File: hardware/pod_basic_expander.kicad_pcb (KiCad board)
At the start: 2 copper layers, 45 x 44 mm, 7 parts, among them J1 POD, SW1 SW_Push, SW2 SW_Push, SW3 SW_Push, SW4 SW_Push

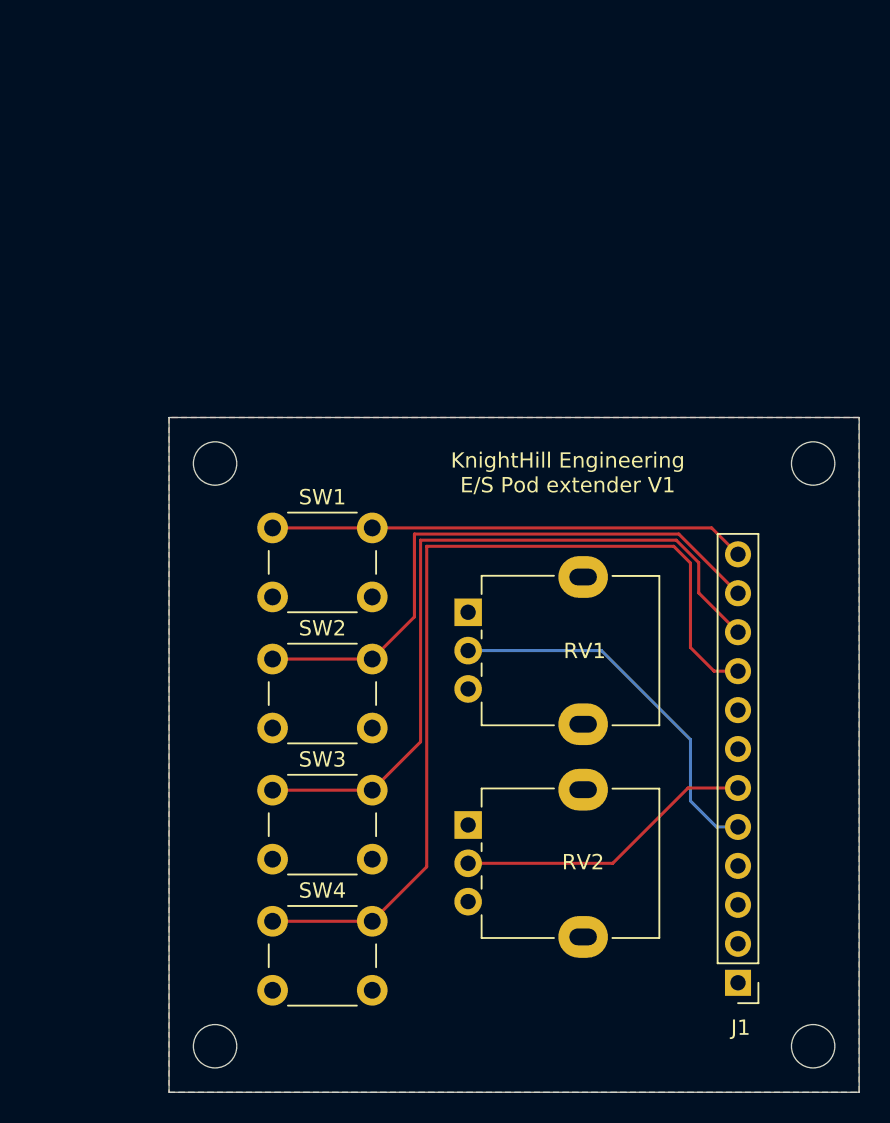
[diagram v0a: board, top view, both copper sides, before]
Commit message: pcd changes
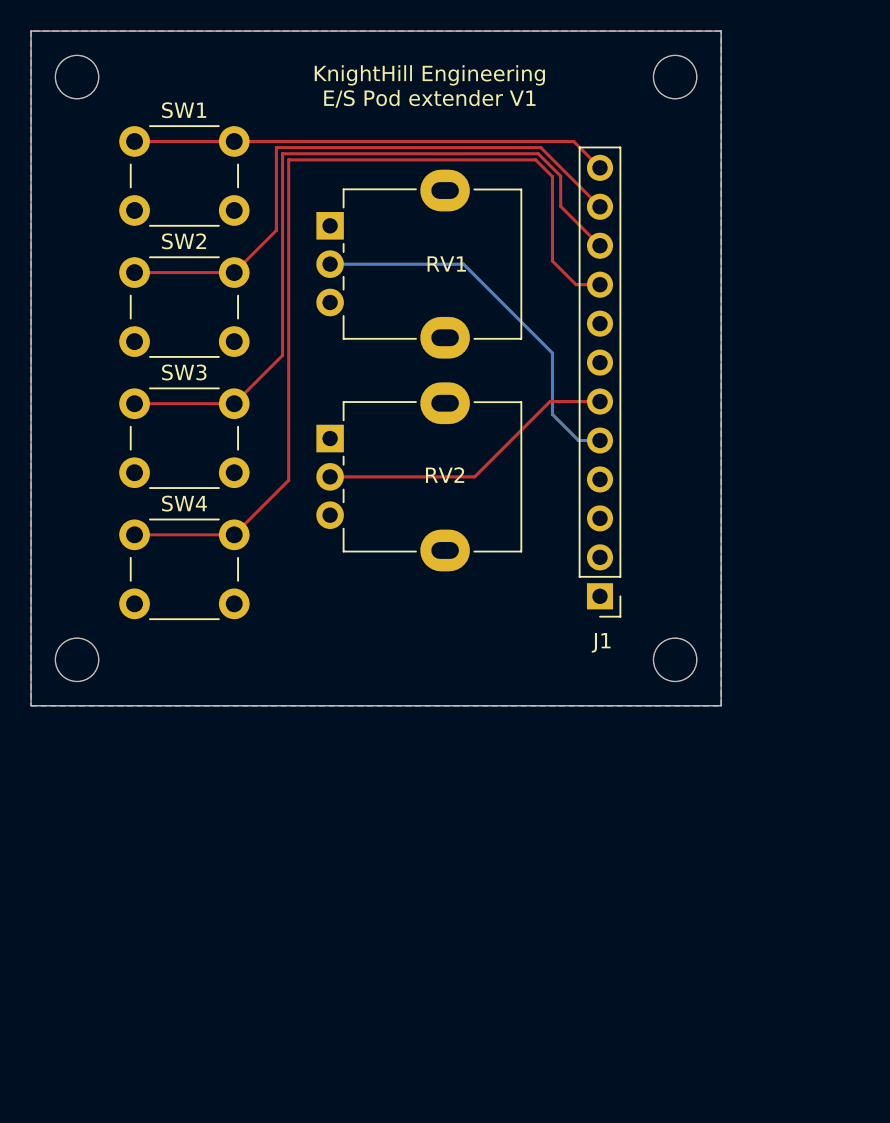
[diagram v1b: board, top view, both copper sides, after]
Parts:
- moved J1 26.8 mm to (101.1, 77.7)
- moved RV1 26.8 mm to (83.5, 53.5)
- moved SW1 26.8 mm to (70.8, 48.0)
- moved SW2 26.8 mm to (70.8, 56.5)
- moved SW3 26.8 mm to (70.8, 65.1)
- moved RV2 26.8 mm to (83.5, 67.4)
- moved SW4 26.8 mm to (70.8, 73.7)
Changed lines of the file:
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@@
   (net 12 "/D7")
   (footprint "Potentiometer_THT:Potentiometer_Alpha_RD901F-40-00D_Single_Vertical" (layer "F.Cu")
-    (at 92.5 92.57)
+    (at 83.5 67.37)
     (descr "Potentiometer, vertical, 9mm, single, http://www.taiwanalpha.com.tw/downloads?target=products&id=113")
     (tags "potentiometer vertical 9mm single")
@@
   )
   (footprint "Button_Switch_THT:SW_PUSH_6mm" (layer "F.Cu")
-    (at 79.75 81.75)
+    (at 70.75 56.55)
     (descr "https://www.omron.com/ecb/products/pdf/en-b3f.pdf")
     (tags "tact sw push 6mm")
@@
   )
   (footprint "Connector_PinHeader_2.54mm:PinHeader_1x12_P2.54mm_Vertical" (layer "F.Cu")
-    (at 110.1 102.86 180)
+    (at 101.1 77.66 180)
     (descr "Through hole straight pin header, 1x12, 2.54mm pitch, single row")
     (tags "Through hole pin header THT 1x12 2.54mm single row")
@@
   )
   (footprint "Button_Switch_THT:SW_PUSH_6mm" (layer "F.Cu")
-    (at 79.75 73.2)
+    (at 70.75 48)
     (descr "https://www.omron.com/ecb/products/pdf/en-b3f.pdf")
     (tags "tact sw push 6mm")
@@
   )
   (footprint "Button_Switch_THT:SW_PUSH_6mm" (layer "F.Cu")
-    (at 79.75 90.3)
+    (at 70.75 65.1)
     (descr "https://www.omron.com/ecb/products/pdf/en-b3f.pdf")
     (tags "tact sw push 6mm")
@@
   )
   (footprint "Potentiometer_THT:Potentiometer_Alpha_RD901F-40-00D_Single_Vertical" (layer "F.Cu")
-    (at 92.5 78.7)
+    (at 83.5 53.5)
     (descr "Potentiometer, vertical, 9mm, single, http://www.taiwanalpha.com.tw/downloads?target=products&id=113")
     (tags "potentiometer vertical 9mm single")
@@
   )
   (footprint "Button_Switch_THT:SW_PUSH_6mm" (layer "F.Cu")
-    (at 79.75 98.85)
+    (at 70.75 73.65)
     (descr "https://www.omron.com/ecb/products/pdf/en-b3f.pdf")
     (tags "tact sw push 6mm")
@@
     )
   )
-  (gr_circle (center 76 107) (end 77 108)
+  (gr_circle (center 67 81.8) (end 68 82.8)
     (stroke (width 0.05) (type default)) (fill none) (layer "Edge.Cuts"))
-  (gr_rect (start 73 66) (end 118 110)
+  (gr_rect (start 64 40.8) (end 109 84.8)
     (stroke (width 0.05) (type default)) (fill none) (layer "Edge.Cuts"))
-  (gr_circle (center 115 69) (end 116 70)
+  (gr_circle (center 106 43.8) (end 107 44.8)
     (stroke (width 0.05) (type default)) (fill none) (layer "Edge.Cuts"))
-  (gr_circle (center 115 107) (end 116 108)
+  (gr_circle (center 106 81.8) (end 107 82.8)
     (stroke (width 0.05) (type default)) (fill none) (layer "Edge.Cuts"))
-  (gr_circle (center 76 69) (end 77 70)
+  (gr_circle (center 67 43.8) (end 68 44.8)
     (stroke (width 0.05) (type default)) (fill none) (layer "Edge.Cuts"))
-  (gr_text "KnightHill Engineering\nE/S Pod extender V1\n" (at 99 71) (layer "F.SilkS")
+  (gr_text "KnightHill Engineering\nE/S Pod extender V1\n" (at 90 45.8) (layer "F.SilkS")
     (effects (font (size 1 1) (thickness 0.1)) (justify bottom))
   )
-  (segment (start 107 91) (end 108.7 92.7) (width 0.2) (layer "B.Cu") (net 5))
-  (segment (start 107 87) (end 107 91) (width 0.2) (layer "B.Cu") (net 5))
-  (segment (start 108.7 92.7) (end 110.1 92.7) (width 0.2) (layer "B.Cu") (net 5))
-  (segment (start 101.2 81.2) (end 107 87) (width 0.2) (layer "B.Cu") (net 5))
-  (segment (start 92.5 81.2) (end 101.2 81.2) (width 0.2) (layer "B.Cu") (net 5))
-  (segment (start 110.1 90.16) (end 106.84 90.16) (width 0.2) (layer "F.Cu") (net 6))
-  (segment (start 106.84 90.16) (end 101.93 95.07) (width 0.2) (layer "F.Cu") (net 6))
-  (segment (start 101.93 95.07) (end 92.5 95.07) (width 0.2) (layer "F.Cu") (net 6))
-  (segment (start 89.8 74.4) (end 105.908628 74.4) (width 0.2) (layer "F.Cu") (net 9))
-  (segment (start 86.25 98.85) (end 89.8 95.3) (width 0.2) (layer "F.Cu") (net 9))
-  (segment (start 105.908628 74.4) (end 107 75.491372) (width 0.2) (layer "F.Cu") (net 9))
-  (segment (start 89.8 95.3) (end 89.8 74.4) (width 0.2) (layer "F.Cu") (net 9))
-  (segment (start 108.54 82.54) (end 110.1 82.54) (width 0.2) (layer "F.Cu") (net 9))
-  (segment (start 107 75.491372) (end 107 81) (width 0.2) (layer "F.Cu") (net 9))
-  (segment (start 107 81) (end 108.54 82.54) (width 0.2) (layer "F.Cu") (net 9))
-  (segment (start 79.75 98.85) (end 86.25 98.85) (width 0.2) (layer "F.Cu") (net 9))
-  (segment (start 89.4 87.15) (end 89.4 74) (width 0.2) (layer "F.Cu") (net 10))
-  (segment (start 79.75 90.3) (end 86.25 90.3) (width 0.2) (layer "F.Cu") (net 10))
-  (segment (start 106.074314 74) (end 107.537157 75.462843) (width 0.2) (layer "F.Cu") (net 10))
-  (segment (start 89.4 74) (end 106.074314 74) (width 0.2) (layer "F.Cu") (net 10))
-  (segment (start 107.537157 77.437157) (end 110.1 80) (width 0.2) (layer "F.Cu") (net 10))
-  (segment (start 86.25 90.3) (end 89.4 87.15) (width 0.2) (layer "F.Cu") (net 10))
-  (segment (start 107.537157 75.462843) (end 107.537157 77.437157) (width 0.2) (layer "F.Cu") (net 10))
-  (segment (start 89 73.6) (end 106.24 73.6) (width 0.2) (layer "F.Cu") (net 11))
-  (segment (start 89 79) (end 89 73.6) (width 0.2) (layer "F.Cu") (net 11))
-  (segment (start 79.75 81.75) (end 86.25 81.75) (width 0.2) (layer "F.Cu") (net 11))
-  (segment (start 86.25 81.75) (end 89 79) (width 0.2) (layer "F.Cu") (net 11))
-  (segment (start 106.24 73.6) (end 110.1 77.46) (width 0.2) (layer "F.Cu") (net 11))
-  (segment (start 86.25 73.2) (end 108.38 73.2) (width 0.2) (layer "F.Cu") (net 12))
-  (segment (start 79.75 73.2) (end 86.25 73.2) (width 0.2) (layer "F.Cu") (net 12))
-  (segment (start 108.38 73.2) (end 110.1 74.92) (width 0.2) (layer "F.Cu") (net 12))
+  (segment (start 98 65.8) (end 99.7 67.5) (width 0.2) (layer "B.Cu") (net 5))
+  (segment (start 98 61.8) (end 98 65.8) (width 0.2) (layer "B.Cu") (net 5))
+  (segment (start 99.7 67.5) (end 101.1 67.5) (width 0.2) (layer "B.Cu") (net 5))
+  (segment (start 92.2 56) (end 98 61.8) (width 0.2) (layer "B.Cu") (net 5))
+  (segment (start 83.5 56) (end 92.2 56) (width 0.2) (layer "B.Cu") (net 5))
+  (segment (start 101.1 64.96) (end 97.84 64.96) (width 0.2) (layer "F.Cu") (net 6))
+  (segment (start 97.84 64.96) (end 92.93 69.87) (width 0.2) (layer "F.Cu") (net 6))
+  (segment (start 92.93 69.87) (end 83.5 69.87) (width 0.2) (layer "F.Cu") (net 6))
+  (segment (start 80.8 49.2) (end 96.908628 49.2) (width 0.2) (layer "F.Cu") (net 9))
+  (segment (start 77.25 73.65) (end 80.8 70.1) (width 0.2) (layer "F.Cu") (net 9))
+  (segment (start 96.908628 49.2) (end 98 50.291372) (width 0.2) (layer "F.Cu") (net 9))
+  (segment (start 80.8 70.1) (end 80.8 49.2) (width 0.2) (layer "F.Cu") (net 9))
+  (segment (start 99.54 57.34) (end 101.1 57.34) (width 0.2) (layer "F.Cu") (net 9))
+  (segment (start 98 50.291372) (end 98 55.8) (width 0.2) (layer "F.Cu") (net 9))
+  (segment (start 98 55.8) (end 99.54 57.34) (width 0.2) (layer "F.Cu") (net 9))
+  (segment (start 70.75 73.65) (end 77.25 73.65) (width 0.2) (layer "F.Cu") (net 9))
+  (segment (start 80.4 61.95) (end 80.4 48.8) (width 0.2) (layer "F.Cu") (net 10))
+  (segment (start 70.75 65.1) (end 77.25 65.1) (width 0.2) (layer "F.Cu") (net 10))
+  (segment (start 97.074314 48.8) (end 98.537157 50.262843) (width 0.2) (layer "F.Cu") (net 10))
+  (segment (start 80.4 48.8) (end 97.074314 48.8) (width 0.2) (layer "F.Cu") (net 10))
+  (segment (start 98.537157 52.237157) (end 101.1 54.8) (width 0.2) (layer "F.Cu") (net 10))
+  (segment (start 77.25 65.1) (end 80.4 61.95) (width 0.2) (layer "F.Cu") (net 10))
+  (segment (start 98.537157 50.262843) (end 98.537157 52.237157) (width 0.2) (layer "F.Cu") (net 10))
+  (segment (start 80 48.4) (end 97.24 48.4) (width 0.2) (layer "F.Cu") (net 11))
+  (segment (start 80 53.8) (end 80 48.4) (width 0.2) (layer "F.Cu") (net 11))
+  (segment (start 70.75 56.55) (end 77.25 56.55) (width 0.2) (layer "F.Cu") (net 11))
+  (segment (start 77.25 56.55) (end 80 53.8) (width 0.2) (layer "F.Cu") (net 11))
+  (segment (start 97.24 48.4) (end 101.1 52.26) (width 0.2) (layer "F.Cu") (net 11))
+  (segment (start 77.25 48) (end 99.38 48) (width 0.2) (layer "F.Cu") (net 12))
+  (segment (start 70.75 48) (end 77.25 48) (width 0.2) (layer "F.Cu") (net 12))
+  (segment (start 99.38 48) (end 101.1 49.72) (width 0.2) (layer "F.Cu") (net 12))
   (zone (net 4) (net_name "VDDA") (layer "F.Cu") (hatch edge 0.5)
     (priority 1)
@@
     (polygon
       (pts
-        (xy 73 66)
-        (xy 73 110)
-        (xy 118 110)
-        (xy 118 66)
+        (xy 64 40.8)
+        (xy 64 84.8)
+        (xy 109 84.8)
+        (xy 109 40.8)
       )
     )
@@
     (polygon
       (pts
-        (xy 105.989194 72.56256)
-        (xy 106 89)
-        (xy 112 89)
-        (xy 111.989194 72.56256)
+        (xy 96.989194 47.36256)
+        (xy 97 63.8)
+        (xy 103 63.8)
+        (xy 102.989194 47.36256)
       )
     )
@@
     (polygon
       (pts
-        (xy 73 66)
-        (xy 73 110)
-        (xy 118 110)
-        (xy 118 66)
+        (xy 64 40.8)
+        (xy 64 84.8)
+        (xy 109 84.8)
+        (xy 109 40.8)
       )
     )
